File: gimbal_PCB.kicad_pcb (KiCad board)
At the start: 4 copper layers, 56.8 x 48.2 mm, 65 parts, among them J2 USB_B_Mini, J5 XT60PW-M, U1 STM32F446RETx, U2 SN65HVD230, U3 TPS54302, U4 ME6211C33M5, U5 USBLC6-2SC6, Y1 16MHz

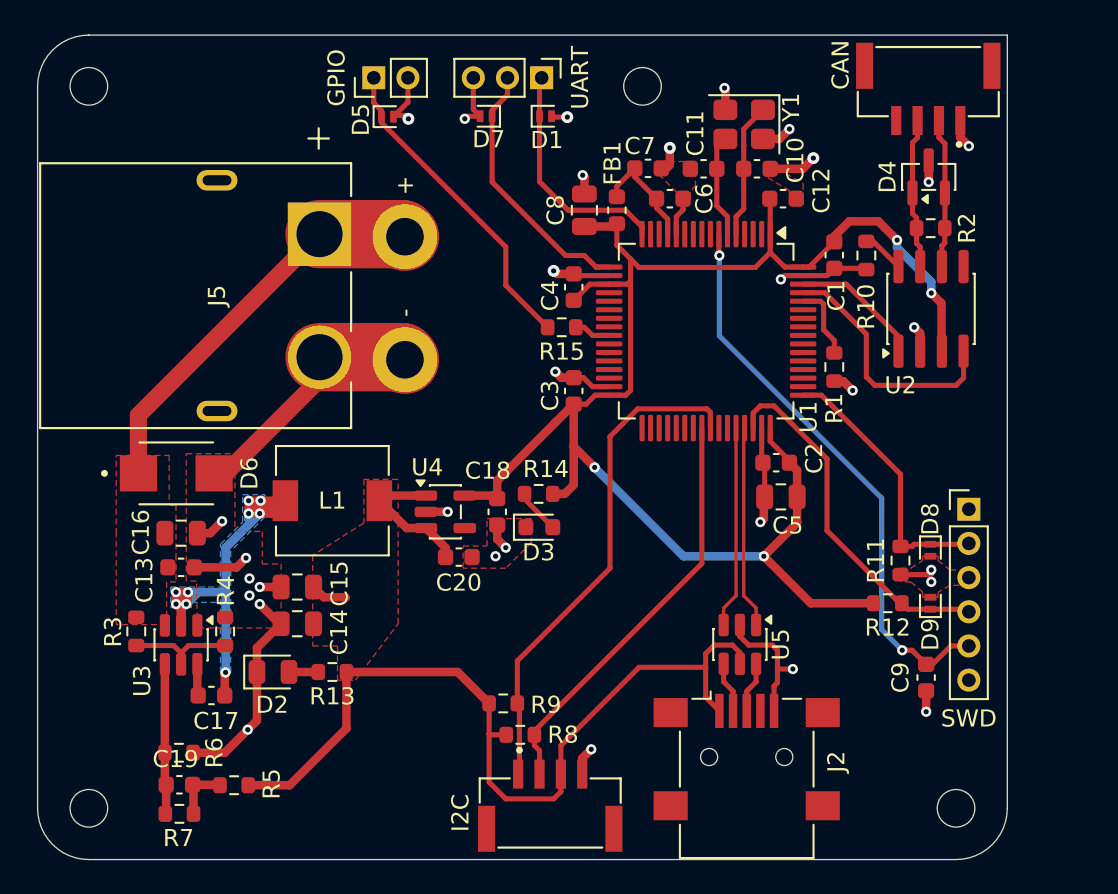
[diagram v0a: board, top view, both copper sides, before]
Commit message: Komplementace a finalni upravy
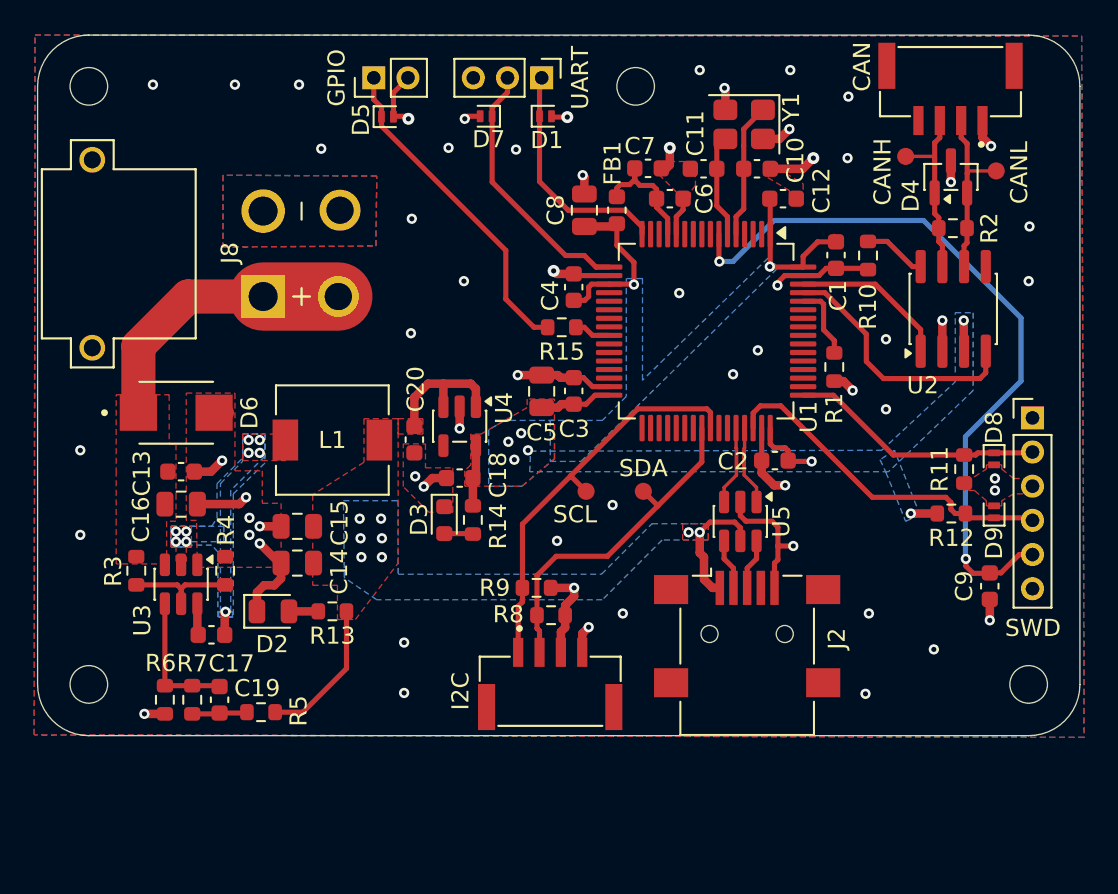
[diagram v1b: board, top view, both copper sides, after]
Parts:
- removed +, -: MountingHole_Pad, MountingHole:MountingHole_2.2mm_M2_DIN965_Pad
- added CANH: Conn_01x01_Pin, Moje_soucastky:Test_point, F.Cu at (80.3, 79.1)
- added CANL: Conn_01x01_Pin, Moje_soucastky:Test_point, F.Cu at (85.6, 80.0)
- added J8: XT30PW-M, XT30PW-M:AMASS_XT30PW-M, F.Cu at (32.7, 84.8)
- added J9: Conn_01x01_Socket, Moje_soucastky:ODrive_PAD, F.Cu at (47.1, 87.3)
- added SCL: Conn_01x01_Pin, Moje_soucastky:Test_point, F.Cu at (61.6, 98.7)
- added SDA: Conn_01x01_Pin, Moje_soucastky:Test_point, F.Cu at (65.0, 98.7)
- J5: value XT60PW-M -> Conn_01x01_Socket; footprint XT60PW-M:AMASS_XT60PW-M -> Moje_soucastky:ODrive_PAD
- moved C5 15.3 mm to (59.0, 92.8), turned to 90 degrees
- moved J5 8.77 mm to (47.2, 82.2), turned to 0 degrees
- moved H4 8.40 mm to (87.5, 110.0)
- moved C20 7.35 mm to (51.5, 95.7), turned to -90 degrees
- moved H5 7.25 mm to (32.5, 110.0)
- moved R8 7.23 mm to (59.5, 106.0), turned to 180 degrees
- moved J2 7.20 mm to (71.0, 107.0)
- moved U5 7.20 mm to (70.6, 100.5)
- moved I2C 7.12 mm to (59.5, 110.4)
- moved R9 7.04 mm to (58.7, 104.3), turned to 180 degrees
- moved R7 6.72 mm to (38.5, 110.9), turned to 90 degrees
- moved D8 6.52 mm to (85.5, 96.8)
- moved C9 6.52 mm to (85.2, 104.2)
- moved D9 6.52 mm to (85.5, 99.9)
- moved R11 6.52 mm to (83.7, 97.4)
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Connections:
- J5 pad 1: napeti_z_baterie -> GND
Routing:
- net +3.3V: track 96.1 -> 34.7 mm, vias 4 -> 9
- net Net-(U3-SW): track 35.5 -> 1.99 mm
- net +5V: track 60.6 -> 30.3 mm, vias 0 -> 9
- net GND: track 91.9 -> 69.4 mm, vias 31 -> 61
- net /NRST: track 33.5 -> 43.0 mm
- net napeti_z_baterie: track 23.5 -> 16.8 mm
- net /USB_D-: track 11.8 -> 5.44 mm
- net /USB_D+: track 11.8 -> 5.59 mm
- net /I2C3_SCL: track 29.6 -> 23.8 mm
- net /I2C3_SDA: track 24.4 -> 20.1 mm
- net Net-(J1-Pin_3): track 8.86 -> 10.6 mm
- net Net-(J1-Pin_2): track 8.77 -> 10.5 mm
- net /CAN1_TX: track 7.72 -> 9.25 mm
- net Net-(U2-Rs): track 3.16 -> 4.36 mm
- net /SWCLK: track 15.9 -> 14.9 mm
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- added copper zone on B.Cu, net +3.3V
- added copper zone on F.Cu, net +3.3V
- added copper zone on B.Cu, net +5V
- added copper zone on B.Cu, net GND
- added copper zone on F.Cu, net Net-(U3-SW)
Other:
- board size 56.8 x 48.2 mm -> 61 x 41 mm
